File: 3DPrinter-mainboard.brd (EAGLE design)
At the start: 109.9 x 74.3 mm, 18 parts, among them J10 Touchscreen, J11 Touchscreen, J31 Power Board, J58 Stepper Driver Board, J6 MicroSD Card

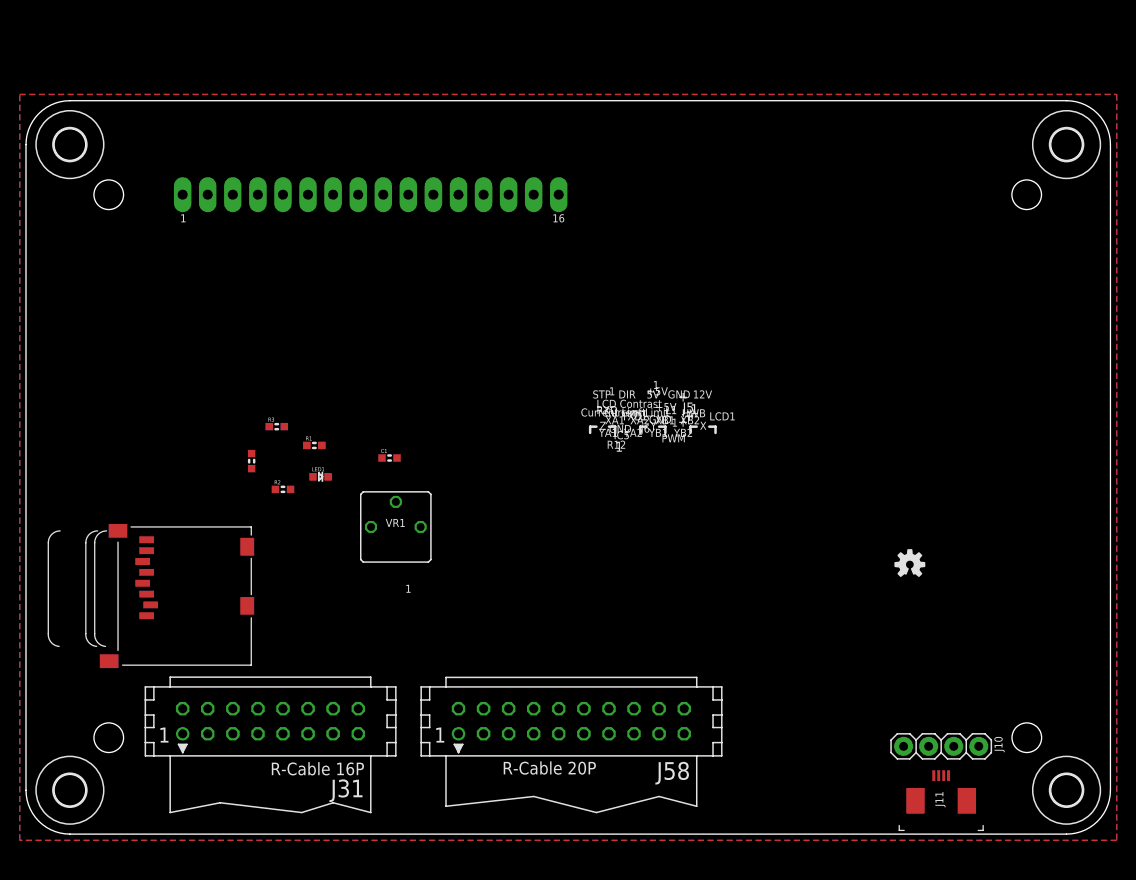
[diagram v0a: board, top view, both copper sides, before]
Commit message: foo
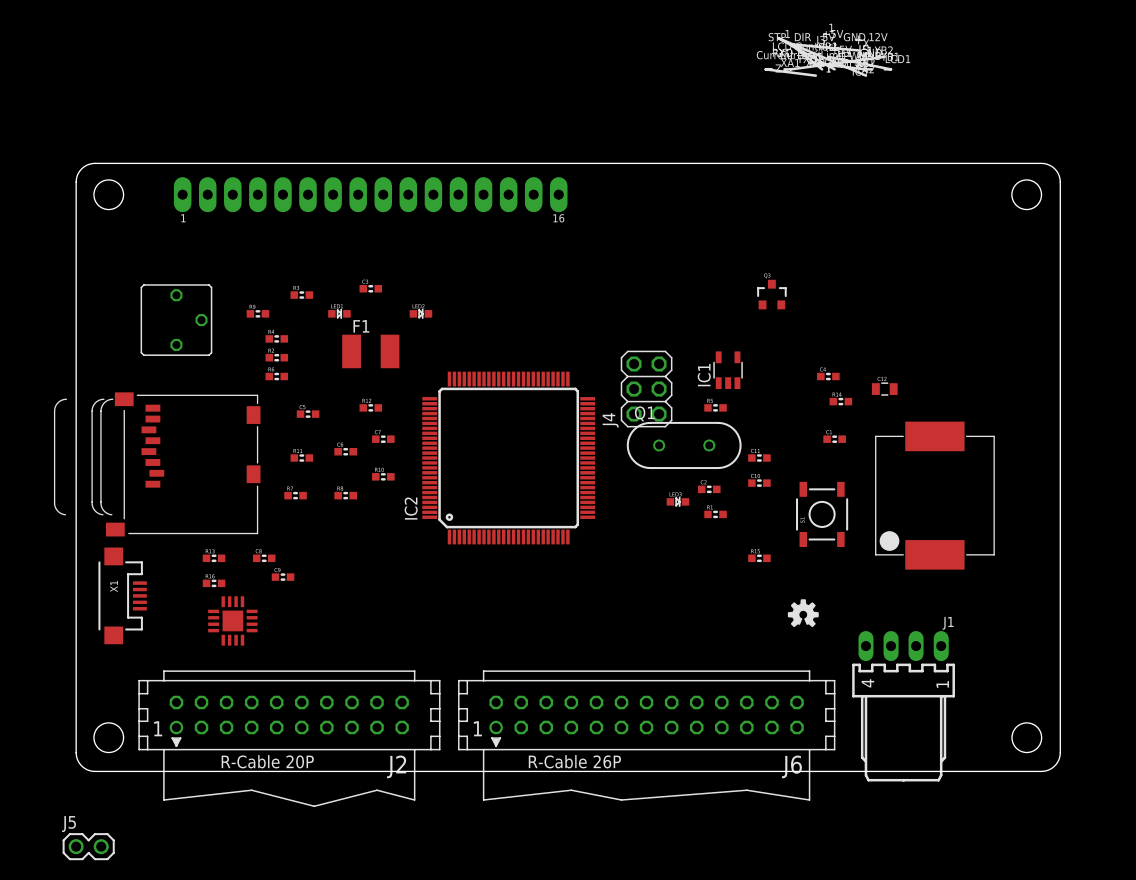
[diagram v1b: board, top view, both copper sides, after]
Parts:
- removed H1, H2, H3, H4: HOLE, holes:3,2
- removed J10: Touchscreen, pinhead:1X04
- removed J11: Touchscreen, SparkFun:DS_TOUCH_CONNECTOR
- removed J31: Power Board, con-harting:CON16L
- removed J58: Stepper Driver Board, con-harting:CON20L
- added C10, C11, C3, C5, C6, C7: 100nF, freetronics-master-v1:0603
- added C12: 4.7µF, freetronics-master-v1:0805
- added C2, C4: 22pF, freetronics-master-v1:0603
- added C8, C9: 47pF, freetronics-master-v1:0603
- added F1: 500mA, freetronics-luke:1812
- added IC1: TL331, linear:DBV-R-PDSO-G5
- added IC2: ATMEGA2560-16AU, atmel-2005:TQFP100
- added IC3: FT230X, serial:QFN4X4-16
- added J1: Encoder, con-molex:7395-04
- added J2: Power Board, con-harting:CON20L
- added J3: MicroSD Card, RAMPSdisplay:ADAFRUIT_MICROSD
- added J4: ISP, freetronics-master-v1:2X03
- added J5: I2C, freetronics-master-v1:1X02
- added LED2: Rx/Grn, freetronics-master-v1:LED-0603
- added LED3: Tx/Yel, freetronics-master-v1:LED-0603
- added Q1: 16MHz, freetronics-master-v1:HC49US
- added Q2: Piezo, RAMPSdisplay:FREETRONICS-MASTER-V1_BUZZER-12X12-SMT
- added Q3: 2N7002, freetronics-master-v1:SOT23-3
- added R10, R14, R15: 1kΩ, freetronics-master-v1:0603
- added R11: 22Ω, freetronics-master-v1:0603
- added R13, R16: 27Ω, freetronics-master-v1:0603
- added R4, R5, R7, R8, R9: 10kΩ, freetronics-master-v1:0603
- added R6: 3.3kΩ, freetronics-master-v1:0603
- added S1: Reset, SparkFun:TACTILE_SWITCH_SMD
- added X1: USB-MICROB, freetronics-master-v1:USB-MICROB
- J6: value MicroSD Card -> Stepper Driver Board; device RAMPSdisplay:ADAFRUIT_MICROSD -> con-harting:CON26L
- R12: value 22Ω -> 10kΩ
- R3: value 1kΩ -> 10kΩ
- moved C1 45.1 mm to (81.9, 40.0)
- moved J6 44.3 mm to (62.9, 12.1), turned to 180 degrees
- moved R1 41.2 mm to (69.8, 32.4)
- moved VR1 30.5 mm to (15.2, 52.1), turned to 90 degrees
- moved LED1 16.6 mm to (31.8, 52.7)
- moved R3 13.6 mm to (27.9, 54.6)
- moved R2 13.4 mm to (25.4, 48.3)
- moved R12 13.2 mm to (34.9, 43.2), turned to 0 degrees
- moved SY 11.9 mm to (78.7, 22.2)
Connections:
- removed net +3.3V: J31.2
- removed net EXTRUDER1_GATE: J31.3
- removed net EXTRUDER2_GATE: J31.4
- removed net LCD_E: LCD1.6
- removed net N$59: LCD1.15, R12.1
- removed net TOUCH1: J10.1, J11.Y1
- removed net TOUCH2: J10.2, J11.X2
- removed net TOUCH3: J10.3, J11.Y2
- removed net TOUCH4: J10.4, J11.X1
- removed net VDD: C1.1, J6.4
- removed net X_LIMIT: J31.13
- removed net Y_LIMIT: J31.14
- removed net Z_LIMIT: J31.15
- new net !RESET: C1.2, IC2.30, J4.5, R5.2, S1.3
- new net +5V: C11.1, C12.1, F1.2, IC3.10, IC3.9
- new net BUZZER: IC1.5, IC2.57
- new net CTS: C1.1, IC3.4
- new net E1_ENABLE: IC2.76, J6.21
- new net E1_GATE: IC2.17, J2.3
- new net E2_ENABLE: IC2.60, J6.22
- new net E2_GATE: IC2.18, J2.4
- new net ENCODER_A: IC2.55, J1.1, R1.2
- new net ENCODER_B: IC2.53, J1.2, R2.2
- new net ENCODER_SWITCH: IC2.78, J1.3, R3.2
- new net LCD_BL: IC2.26, Q3.1, R12.2
- new net LCD_EN: IC2.12, LCD1.6
- new net N$1: LCD1.16, R11.1
- new net N$10: IC3.11, R15.2
- new net N$11: LED2.C, R14.1
- new net N$12: IC3.5, R14.2
- new net N$2: LED3.C, R15.1
- new net N$3: Q3.3, R11.2
- new net N$30: C3.1, IC1.1, R6.2
- new net N$31: IC1.3, R4.2, R7.2
- new net N$34: IC1.4, Q2.2, R4.1, R6.1
- new net N$36: C4.2, IC2.34, Q1.1
- new net N$37: C10.1, IC3.1, IC3.8
- new net N$38: C6.1, IC2.98
- new net N$39: IC3.6, R16.1
- new net N$4: IC3.7, R13.1
- new net N$40: C8.1, R16.2, X1.D+
- new net N$41: C9.1, R13.2, X1.D-
- new net N$52: F1.1, X1.VBUS
- new net N$8: C2.2, IC2.33, Q1.2
- new net RXD0: IC2.2, IC3.15
- new net SCL: IC2.43, J5.2
- new net SDA: IC2.44, J5.1
- new net TXD0: IC2.3, IC3.2
- new net X_ENABLE: IC2.50, J6.18
- new net X_MAX: IC2.6, J2.14
- new net X_MIN: IC2.7, J2.13
- new net Y_ENABLE: IC2.24, J6.19
- new net Y_MAX: IC2.63, J2.16
- new net Y_MIN: IC2.64, J2.15
- new net Z_ENABLE: IC2.25, J6.20
- new net Z_MAX: IC2.45, J2.18
- new net Z_MIN: IC2.46, J2.17
- net !SD_CS: now also IC2.42, J3.2, R10.2, R8.2; no longer J6.2, R2.2, R3.2
- net !SD_DETECT: now also IC2.51, J3.CD1, R9.2; no longer J6.CD1, R1.2
- net !TC1_CS: now also IC2.41, J2.8; no longer J31.8
- net !TC2_CS: now also IC2.40, J2.9; no longer J31.9
- net !TC3_CS: now also IC2.39, J2.10; no longer J31.10
- net +24V: now also J6.24, J6.26; no longer J58.20
- net +3V3: now also C5.1, C7.1, IC2.10, IC2.100, IC2.31, IC2.61, IC2.80, J2.19, J2.20, J3.4, J4.2, J6.23, J6.25, LCD1.15, LED2.A, LED3.A, R12.1, R3.1, R5.1, R8.1, R9.1; no longer J58.18, J58.2, R12.2
- net BEDHEATER_GATE: now also IC2.23, J2.5; no longer J31.5
- net E1_DIR: now also IC2.72, J6.9; no longer J58.10
- net E1_STEP: now also IC2.74, J6.10; no longer J58.9
- net E1_VREF: now also IC2.94, J6.16; no longer J58.16
- net E2_DIR: now also IC2.56, J6.11; no longer J58.12
- net E2_STEP: now also IC2.54, J6.12; no longer J58.11
- net E2_VREF: now also IC2.93, J6.17; no longer J58.17
- net FAN1_GATE: now also IC2.70, J2.6; no longer J31.6
- net FAN2_GATE: now also IC2.52, J2.7; no longer J31.7
- net GND: now also C10.2, C11.2, C12.2, C2.1, C3.2, C4.1, C5.2, C6.2, C7.2, C8.2, C9.2, IC1.2, IC2.11, IC2.32, IC2.62, IC2.81, IC2.99, IC3.13, IC3.3, IC3.C, J1.4, J2.1, J2.2, J3.6, J3.MT1, J3.MT2, J4.6, J6.1, J6.2, Q2.1, Q3.2, R7.1, S1.1, X1.GND; no longer C1.2, J31.1, J31.16, J58.1, J58.19, J6.6, J6.MT1, J6.MT2, LCD1.16
- net LCD_D4: now also IC2.77
- net LCD_D5: now also IC2.75
- net LCD_D6: now also IC2.73
- net LCD_D7: now also IC2.71
- net LCD_RS: now also IC2.13
- net MISO: now also IC2.22, J2.11, J3.7, J4.1; no longer J31.11, J6.7
- net MOSI: now also IC2.21, J3.3, J4.4; no longer J6.3
- net N$13: now also R10.1; no longer R3.1
- net SCK: now also IC2.20, J2.12, J3.5, J4.3; no longer J31.12, J6.5
- net X_DIR: now also IC2.5, J6.3; no longer J58.4
- net X_STEP: now also IC2.1, J6.4; no longer J58.3
- net X_VREF: now also IC2.97, J6.13; no longer J58.13
- net Y_DIR: now also IC2.16, J6.5; no longer J58.6
- net Y_STEP: now also IC2.15, J6.6; no longer J58.5
- net Y_VREF: now also IC2.96, J6.14; no longer J58.14
- net Z_DIR: now also IC2.58, J6.7; no longer J58.8
- net Z_STEP: now also IC2.59, J6.8; no longer J58.7
- net Z_VREF: now also IC2.95, J6.15; no longer J58.15
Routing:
- removed copper zone on layer 1, net GND
- removed copper zone on layer 16, net GND
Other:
- board size 109.9 x 74.3 mm -> 99.7 x 61.6 mm
